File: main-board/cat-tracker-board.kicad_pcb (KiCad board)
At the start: 2 copper layers, 51.7 x 23.1 mm, 31 parts, among them J1 Conn_01x10, J3 USB_B_Micro, Q1 SI3443DDV-T1-GE3, SW1 PCM12SMTR, U1 ATSAMD21E18A-M, U3 L80-R, U4 RFM95W-915S2, U5 MCP73831-2ACI/MC, U6 MCP1700T-3602E/TT

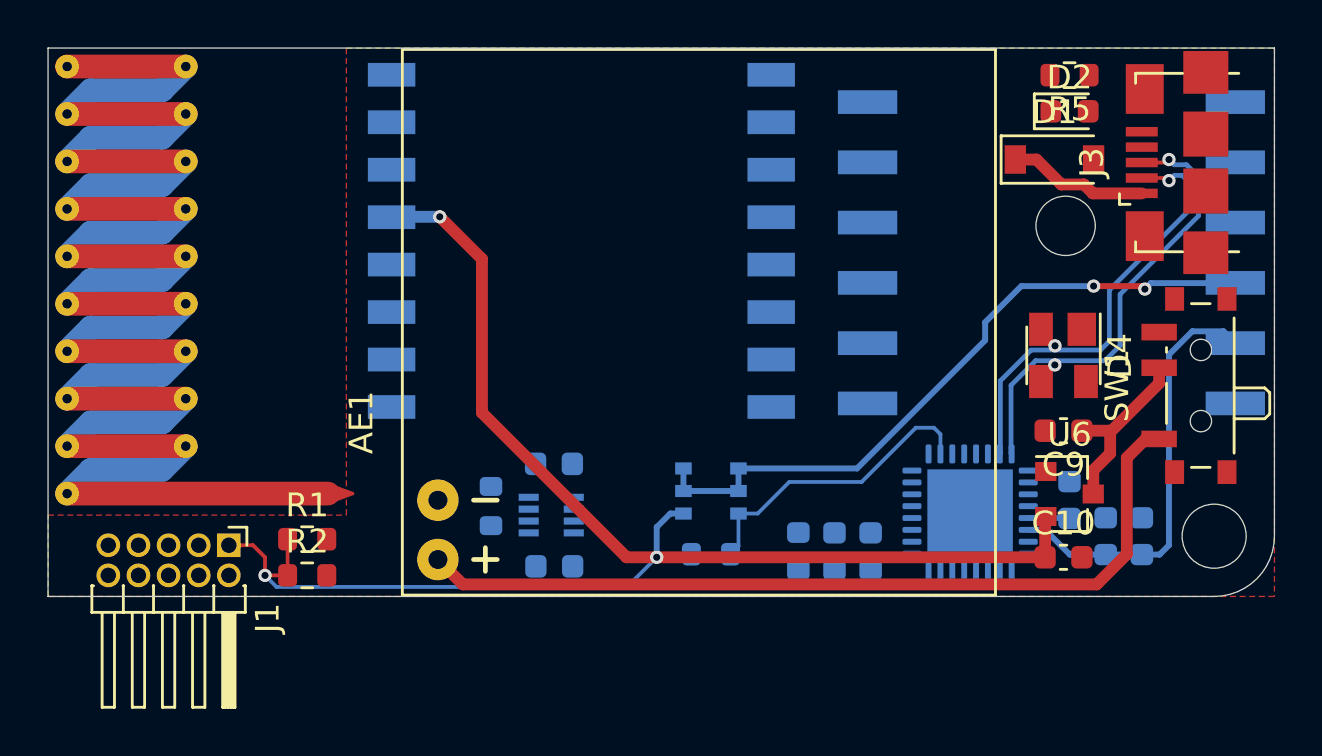
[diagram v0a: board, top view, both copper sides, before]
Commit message: Work on layout.
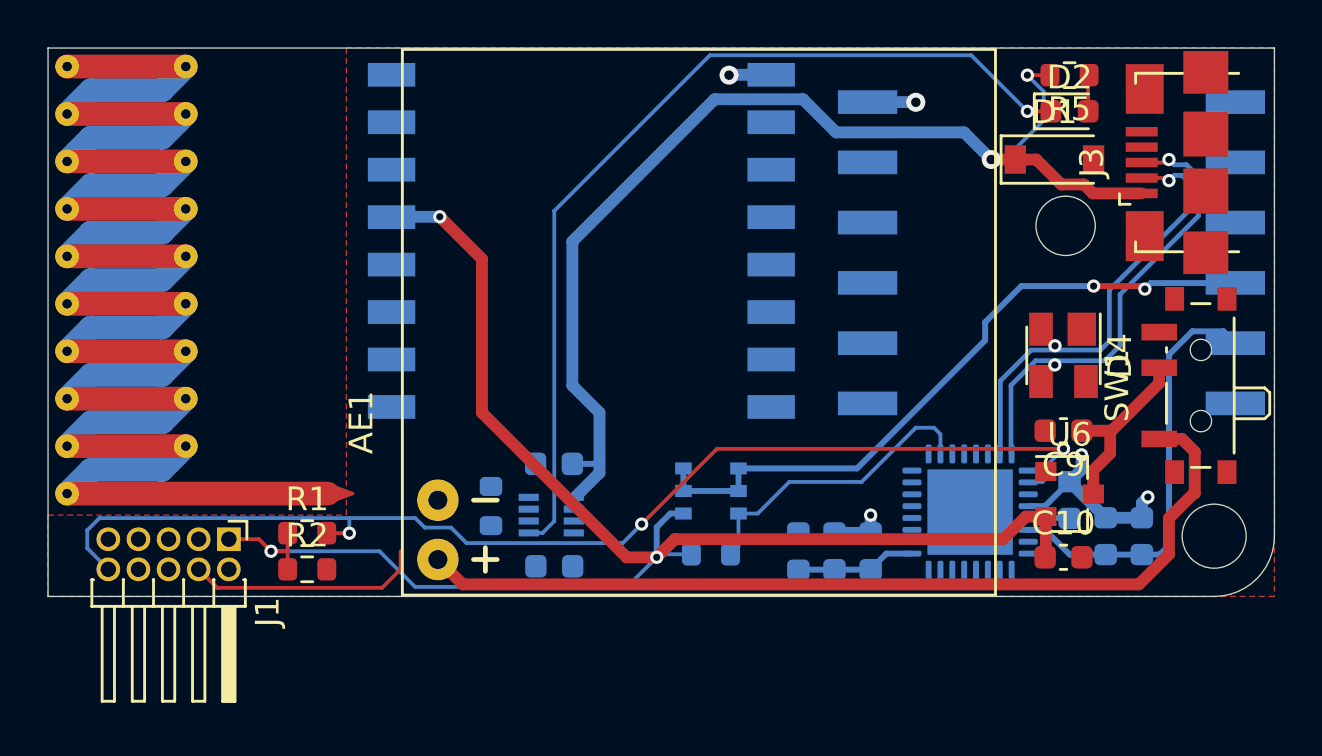
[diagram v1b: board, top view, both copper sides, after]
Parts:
- moved R1 0.25 mm to (10.9, 20.4)
- moved R2 0.25 mm to (10.9, 22.0)
- moved J1 0.25 mm to (7.62, 20.7)
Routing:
- net /nRESET: track 0.00 -> 49.4 mm, vias 0 -> 3
- net /VUSB: track 5.92 -> 47.5 mm, vias 0 -> 2
- net Net-(D2-Pad1): track 0.00 -> 39.0 mm, vias 0 -> 1
- net /GND: track 0.00 -> 16.2 mm, vias 0 -> 5
- net /SWCLK: track 0.00 -> 9.92 mm
- net Net-(C4-Pad1): track 0.00 -> 5.08 mm
- net /VBAT: track 35.8 -> 38.3 mm
- net Net-(D2-Pad2): track 0.00 -> 1.54 mm
